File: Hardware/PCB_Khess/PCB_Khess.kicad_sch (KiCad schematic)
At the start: 13 parts, among them J1 Screw_Terminal_01x02, J2 USB3_A, J3 RJ11_Connector, J4 Conn_01x02, Q1 IRF540NPBF, U1 R-78B5.0-2.0

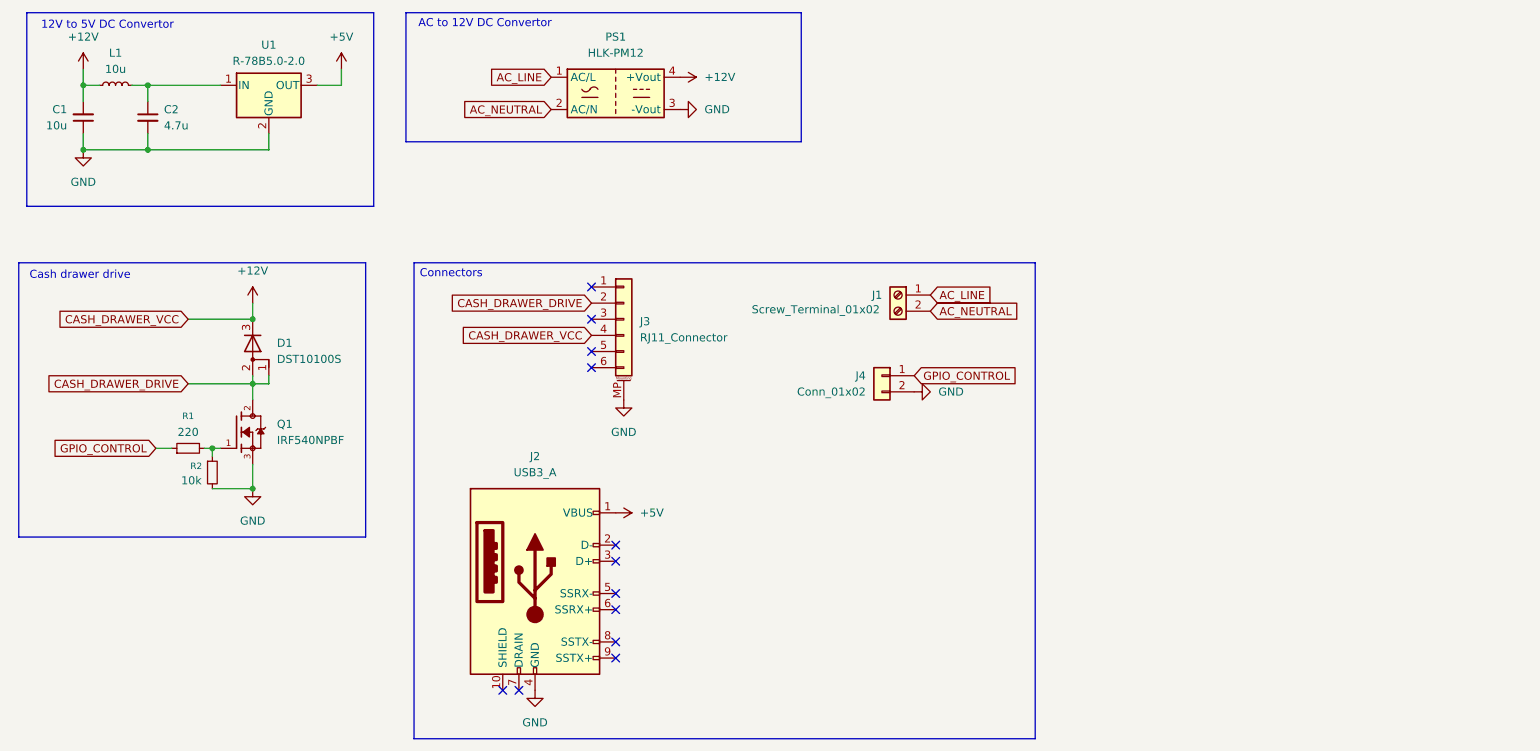
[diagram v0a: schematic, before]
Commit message: fix: update pcb main
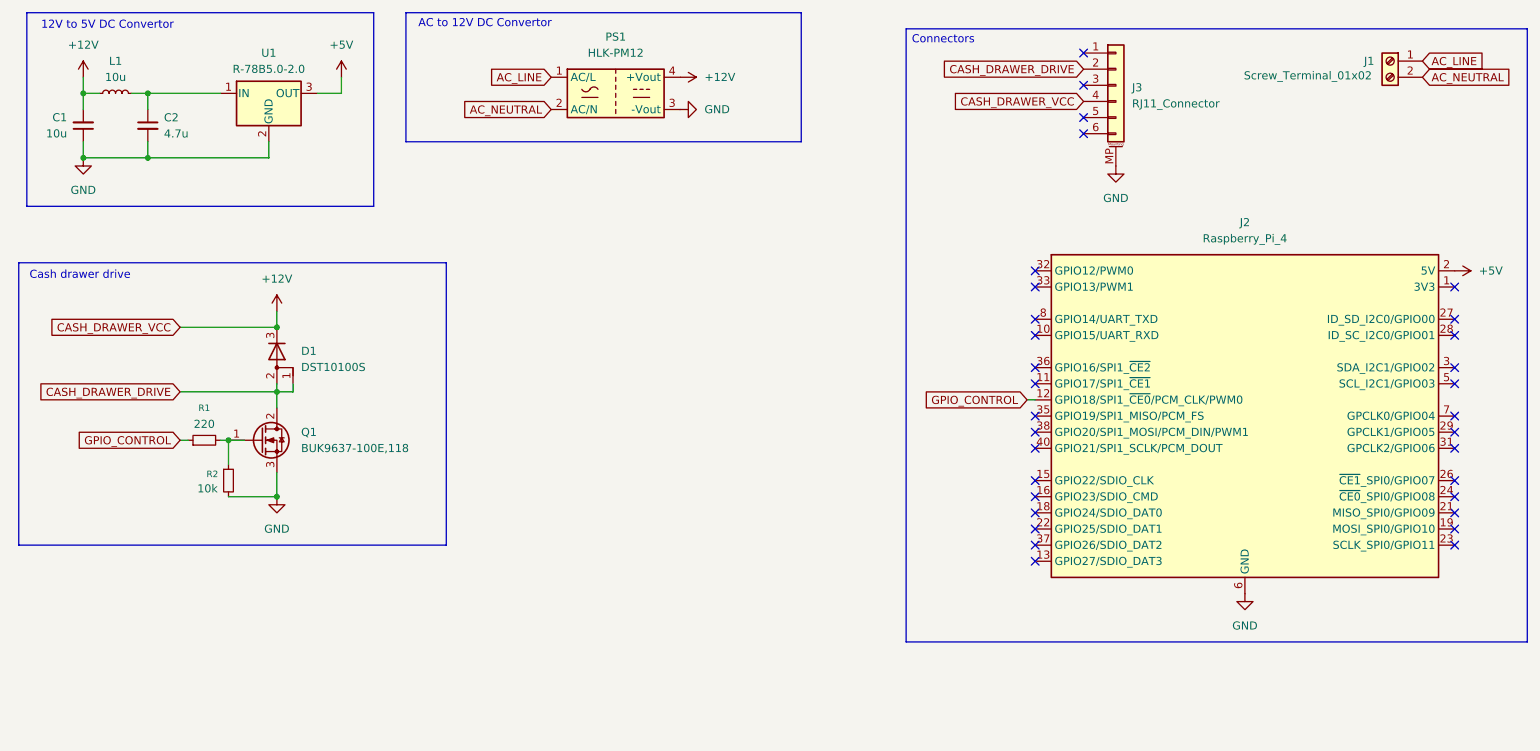
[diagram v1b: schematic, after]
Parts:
- removed J2: USB3_A, symbol Connector:USB3_A
- removed J4: Conn_01x02, symbol Connector_Generic:Conn_01x02
- removed Q1: IRF540NPBF, IRF540NPBF:TO254P1054X469X1930-3, symbol IRF540NPBF:IRF540NPBF
- added J2: Raspberry_Pi_4, symbol Connector:Raspberry_Pi_4
- added Q1: BUK9637-100E,118, symbol Transistor_FET:Q_NMOS_GDS
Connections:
- net +5V: now also J2.2 (5V), J2.4 (5V)
- net CASH_DRAWER_DRIVE: now also Q1.2 (D)
- net GND: now also J2.14 (GND), J2.20 (GND), J2.25 (GND), J2.30 (GND), J2.34 (GND), J2.39 (GND), J2.6 (GND), J2.9 (GND), Q1.3 (S)
- net GPIO_CONTROL: now also J2.12 (GPIO18/SPI1_~{CE0}/PCM_CLK/PWM0)
- net at R1.2, R2.1: now also Q1.1 (G)
- new net: J2.1 (3V3), J2.17 (3V3)
- no-connect marks 12 -> 32
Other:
- moved on the sheet: C1, C2, D1, J1, J3, L1, R1, R2, U1
